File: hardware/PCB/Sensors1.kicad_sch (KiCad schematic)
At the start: 22 parts, among them J10 WCS1800, J101 INA333, J11 INA333, Q2 IRLZ44N, U102 INA333xxDGK, U103 LM358, U201 QNHC3, U4 LM358

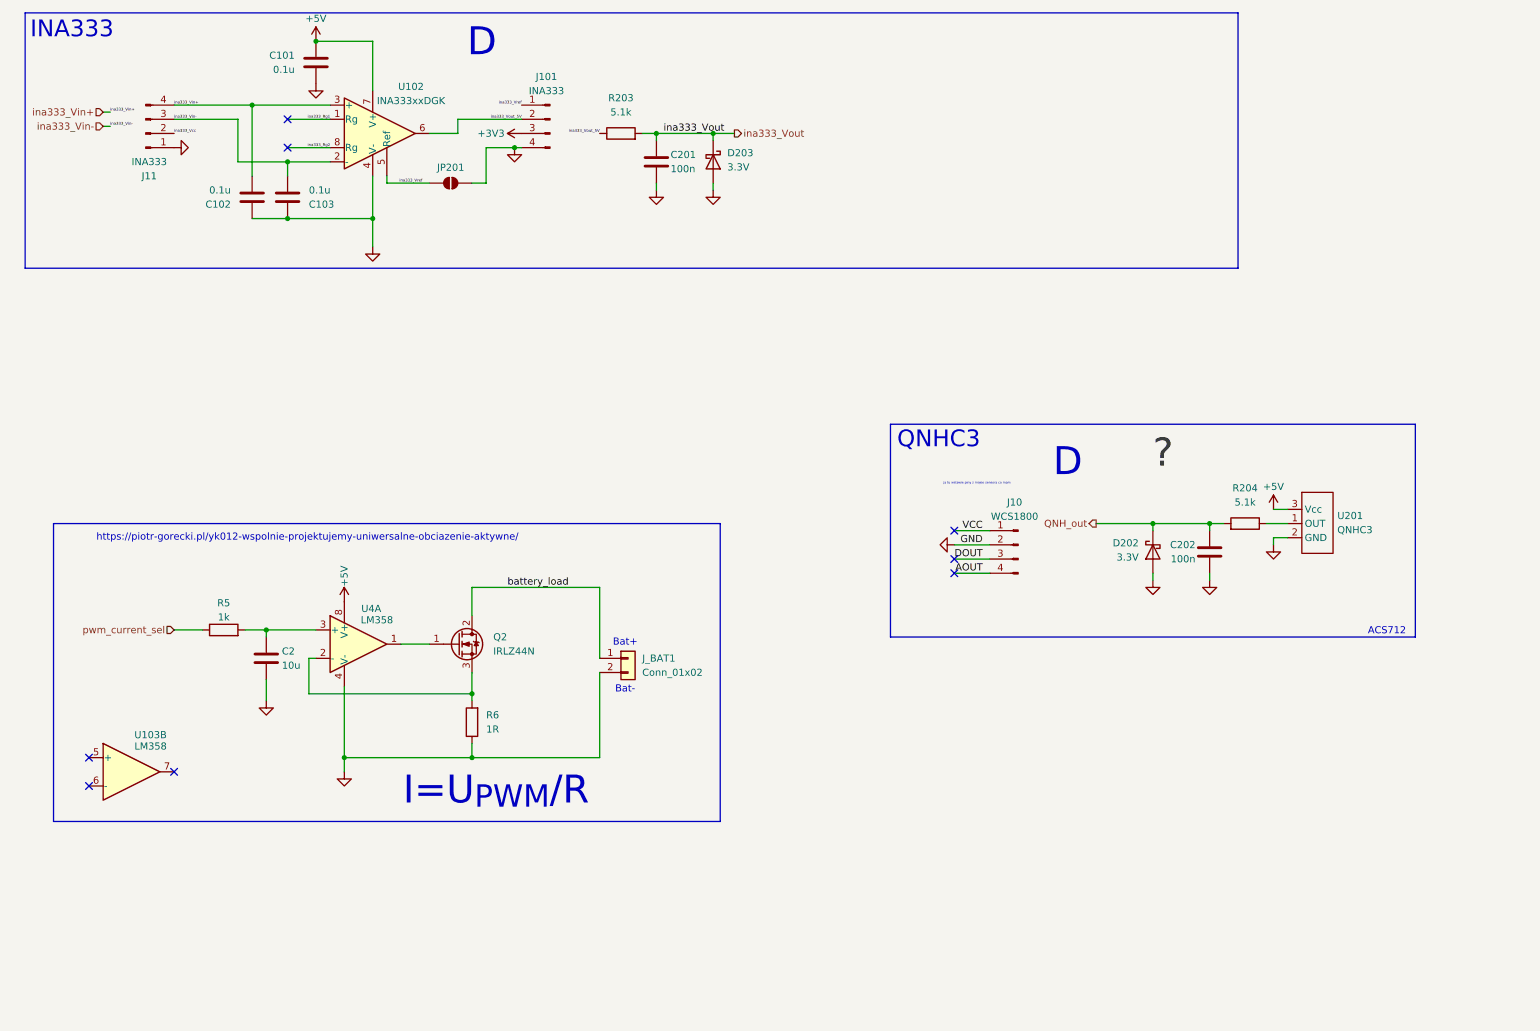
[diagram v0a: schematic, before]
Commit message: PCB
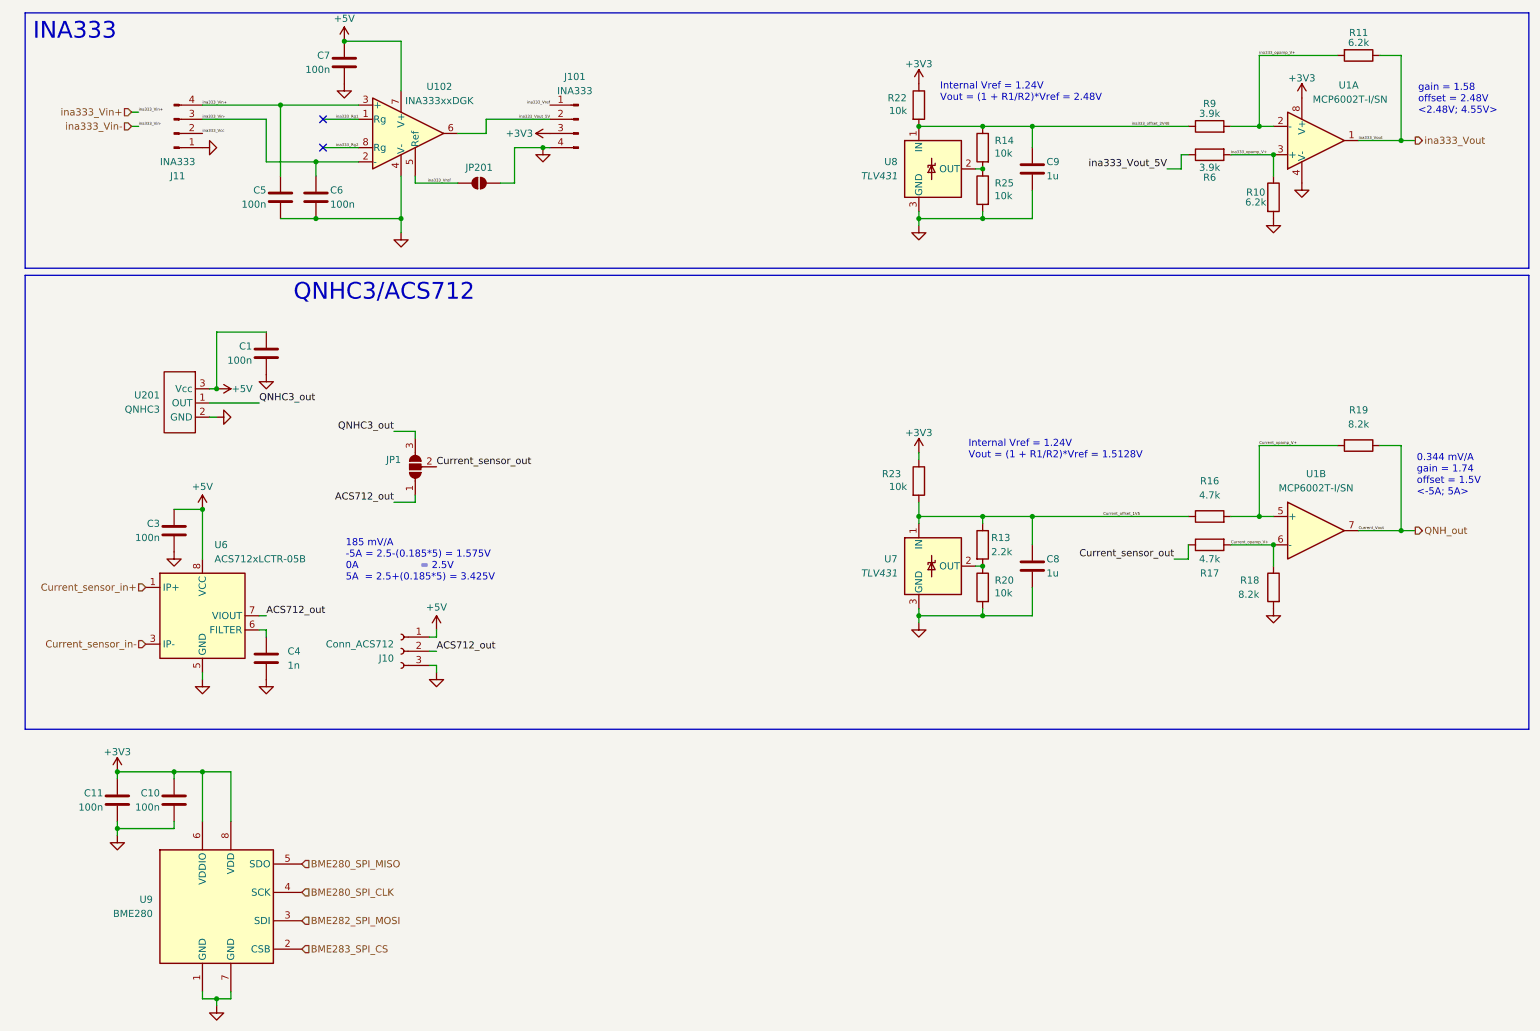
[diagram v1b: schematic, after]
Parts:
- removed C101, C102, C103: 0.1u, Capacitor_SMD:C_0805_2012Metric, symbol Device:C
- removed C2: 10u, Capacitor_SMD:C_1206_3216Metric, symbol Device:C
- removed C201, C202: 100n, Capacitor_SMD:C_0805_2012Metric, symbol Device:C
- removed D202, D203: 3.3V, Diode_SMD:D_SOD-323, symbol Device:D_Schottky
- removed J10: WCS1800, Connector_PinHeader_2.54mm:PinHeader_1x04_P2.54mm_Vertical, symbol Connector:Conn_01x04_Pin
- removed J_BAT1: Conn_01x02, TerminalBlock:TerminalBlock_MaiXu_MX126-5.0-02P_1x02_P5.00mm, symbol Connector_Generic:Conn_01x02
- removed Q2: IRLZ44N, Package_TO_SOT_THT:TO-220-3_Vertical, symbol Transistor_FET:IRLZ44N
- removed R203, R204: 5.1k, Resistor_SMD:R_0805_2012Metric, symbol Device:R
- removed R5: 1k, Resistor_SMD:R_0805_2012Metric, symbol Device:R
- removed U103, U4: LM358, footprints:LM358, symbol Amplifier_Operational:LM358
- added C1, C10, C11, C3, C5, C6, C7: 100n, Capacitor_SMD:C_0805_2012Metric, symbol Device:C
- added C4: 1n, Capacitor_SMD:C_0805_2012Metric, symbol Device:C
- added C8, C9: 1u, Capacitor_SMD:C_0805_2012Metric, symbol Device:C
- added J10: Conn_ACS712, symbol Connector:Conn_01x03_Socket
- added JP1: SolderJumper_3_Open, Jumper:SolderJumper-3_P2.0mm_Open_TrianglePad1.0x1.5mm_NumberLabels, symbol Jumper:SolderJumper_3_Open
- added R10, R11: 6.2k, Resistor_SMD:R_0805_2012Metric, symbol Device:R
- added R13: 2.2k, Resistor_SMD:R_0805_2012Metric, symbol Device:R
- added R14, R20, R22, R23, R25: 10k, Resistor_SMD:R_0805_2012Metric, symbol Device:R
- added R16, R17: 4.7k, Resistor_SMD:R_0805_2012Metric, symbol Device:R
- added R18, R19: 8.2k, Resistor_SMD:R_0805_2012Metric, symbol Device:R
- added R9: 3.9k, Resistor_SMD:R_0805_2012Metric, symbol Device:R
- added U1: MCP6002T-I/SN, Package_SO:SOIC-8_3.9x4.9mm_P1.27mm, symbol Amplifier_Operational:MCP6002-xSN
- added U6: ACS712xLCTR-05B, Package_SO:SOIC-8_3.9x4.9mm_P1.27mm, symbol Sensor_Current:ACS712xLCTR-05B
- added U7, U8: TLV431, Package_TO_SOT_SMD:SOT-23, symbol Reference_Voltage:REF3012
- added U9: BME280, Package_LGA:Bosch_LGA-8_2.5x2.5mm_P0.65mm_ClockwisePinNumbering, symbol Sensor:BME280
- R6: value 1R -> 3.9k; footprint (none) -> Resistor_SMD:R_0805_2012Metric; JLCPCB Part (none) -> C17614; Link (none) -> https://jlcpcb.com/partdetail/18302-0805W8F3901T5E/C17614; MFR Part (none) -> 0805W8F3901T5E; Manufacturer (none) -> UNI-ROYAL(Uniroyal Elec); now in the parts list
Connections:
- net +3V3: now also C10.1, C11.1, R22.1, R23.1, U1.8 (V+), U9.6 (VDDIO), U9.8 (VDD)
- net +5V: now also C1.1, C3.1, C7.1, J10.1 (Pin_1), U6.8 (VCC)
- net GND: now also C1.2, C10.2, C11.2, C3.2, C4.2, C5.2, C6.2, C7.2, C8.2, C9.2, J10.3 (Pin_3), R10.2, R18.2, R20.2, R25.2, U1.4 (V-), U6.5 (GND), U7.3 (GND), U8.3 (GND), U9.1 (GND), U9.7 (GND); no longer R6.1
- net QNH_out: now also R19.1, U1.7
- net ina333_Vin+: now also C5.1
- net ina333_Vin-: now also C6.1
- net ina333_Vout: now also R11.1, U1.1
- net ina333_Vout_5V: now also R6.1
- net ina333_opamp_V+: now reaches R6.2
- net ina333_opamp_V+: now also R10.1, R11.2, R9.2, U1.2 (-), U1.3 (+)
- net QNHC3_out: now reaches U201.1 (OUT)
- net QNHC3_out: now also JP1.3 (B)
- new net: R14.2, R25.1, U8.2 (OUT)
- new net: R13.2, R20.1, U7.2 (OUT)
- new net: C4.1, U6.6 (FILTER)
- new net ACS712_out: J10.2 (Pin_2), JP1.1 (A), U6.7 (VIOUT)
- new net BME280_SPI_CLK: U9.4 (SCK)
- new net BME280_SPI_MISO: U9.5 (SDO)
- new net BME282_SPI_MOSI: U9.3 (SDI)
- new net BME283_SPI_CS: U9.2 (CSB)
- new net Current_offset_1V5: C8.1, R13.1, R16.1, R23.2, U7.1 (IN)
- new net Current_opamp_V+: R16.2, R17.2, R18.1, R19.2, U1.5 (+), U1.6 (-)
- new net Current_sensor_in+: U6.1 (IP+), U6.2 (IP+)
- new net Current_sensor_in-: U6.3 (IP-), U6.4 (IP-)
- new net Current_sensor_out: JP1.2 (C), R17.1
- new net ina333_offset_2V48: C9.1, R14.1, R22.2, R9.1, U8.1 (IN)
- no-connect marks 8 -> 2
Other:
- note added: "0.344 mV/A gain = 1.74 offset = 1.5V <-5A; 5A>"
- note added: "185 mV/A -5A = 2.5-(0.185*5) = 1.575V 0A = 2.5V 5A = 2.5+(0.185*5) = 3.425V"
- note added: "Internal Vref = 1.24V Vout = (1 + R1/R2)*Vref = 1.5128V"
- note added: "Internal Vref = 1.24V Vout = (1 + R1/R2)*Vref = 2.48V"
- note added: "QNHC3/ACS712"
- note added: "gain = 1.58 offset = 2.48V <2.48V; 4.55V>"
- note removed: "ACS712"
- note removed: "Bat+"
- note removed: "Bat-"
- note removed: "D"
- note removed: "I=U_{PWM}/R"
- note removed: "QNHC3"
- note removed: "https://piotr-gorecki.pl/yk012-wspolnie-projektujemy-uniwersalne-obciazenie-aktywne/"
- note removed: "ja tu wstawie piny z mojeo sensora co mam"
- moved on the sheet: J101, J11, JP201, U102, U201
